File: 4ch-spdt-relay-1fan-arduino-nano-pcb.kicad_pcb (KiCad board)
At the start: 2 copper layers, 143.9 x 97.2 mm, 54 parts, among them J1 Screw_Terminal_01x03, J2 Conn_01x08_Pin, J3 Screw_Terminal_01x03, J4 Screw_Terminal_01x03, J5 Screw_Terminal_01x03, J7 Conn_01x07_Pin, J9 Conn_01x04_Pin, K1 G5LE-1, K2 G5LE-1, K3 G5LE-1, K4 G5LE-1, Q1 2N3904, Q2 2N3904, Q3 2N3904, Q4 2N3904, Q5 BT136, U5 MOC3021M, U6 PC817, U7 TSOP1738, U8 HLK-10M05

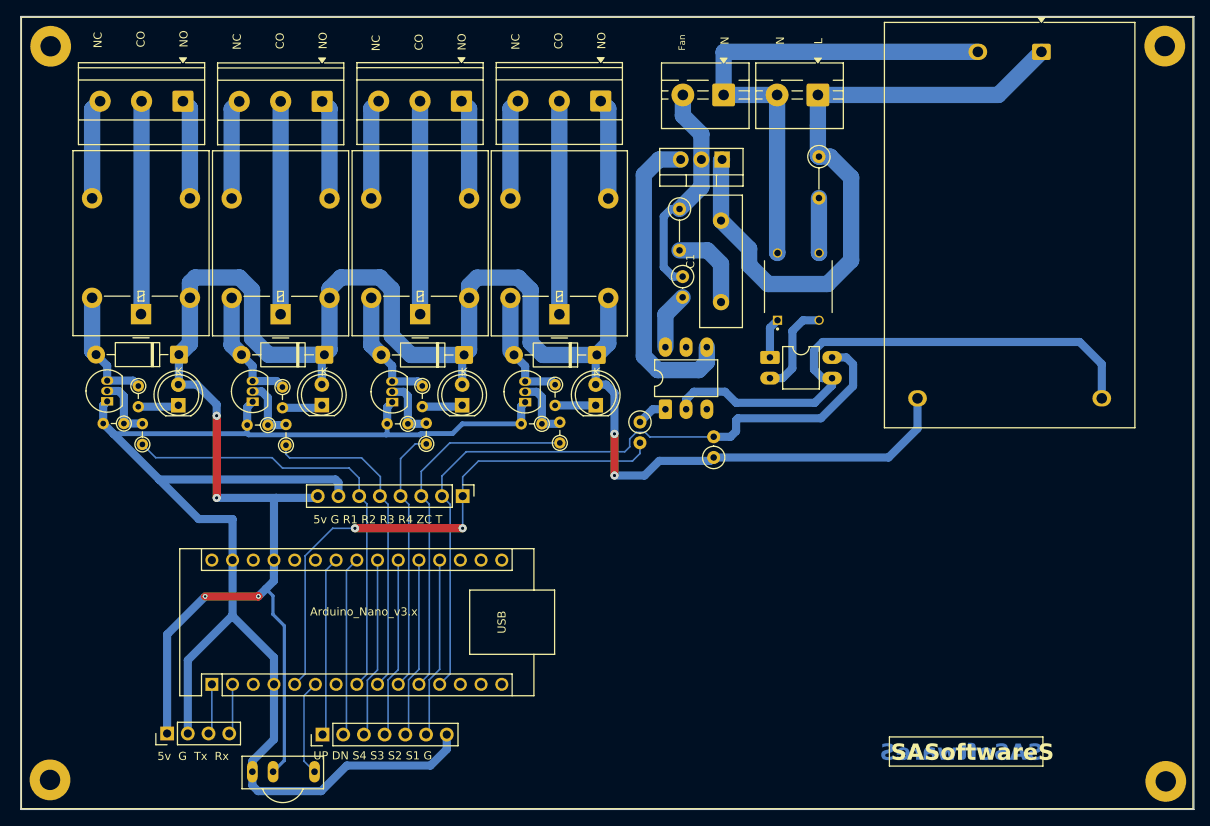
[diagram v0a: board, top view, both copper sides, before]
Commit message: Add files via upload
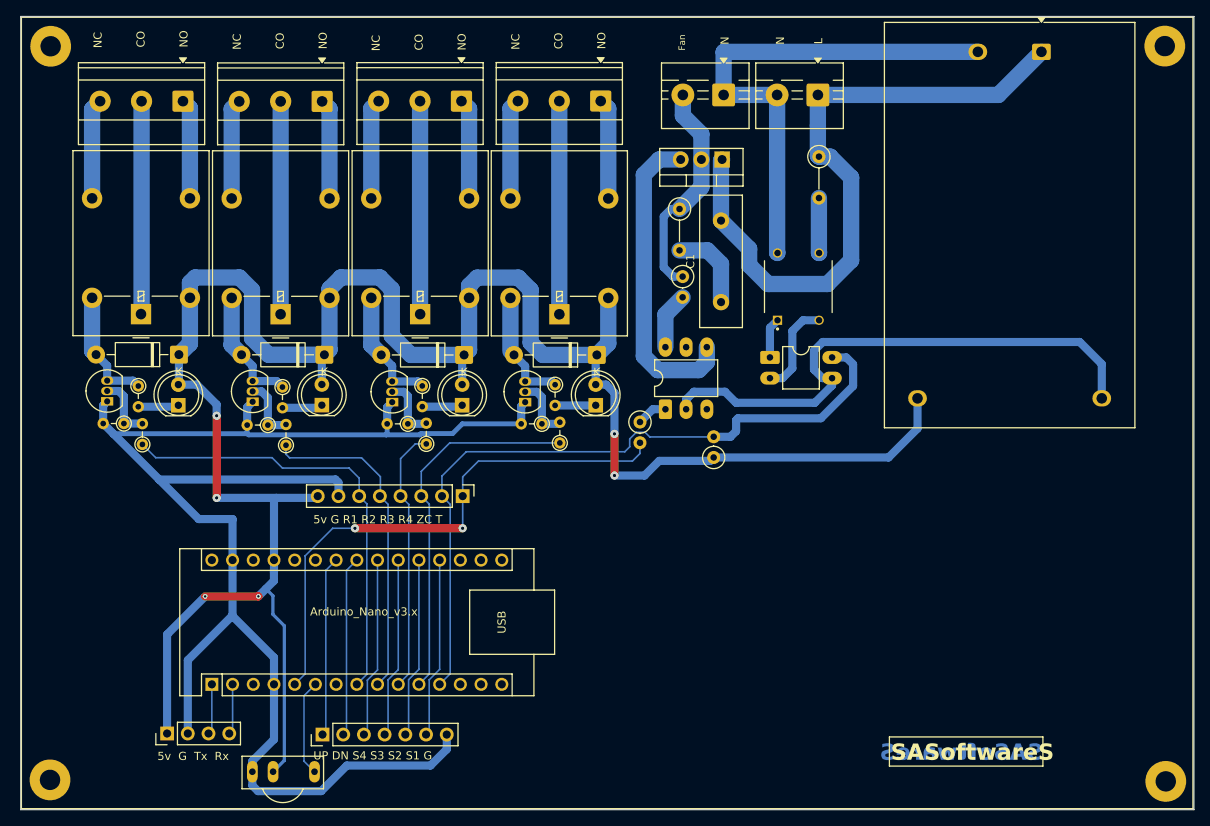
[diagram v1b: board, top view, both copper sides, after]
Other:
- board size 143.9 x 97.2 mm -> 143.9 x 97.3 mm
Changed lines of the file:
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@@
 		(model "${KICAD10_3DMODEL_DIR}/Module.3dshapes/Arduino_Nano.STEP"
 			(offset
-				(xyz 7.5 -17.5 0)
+				(xyz 7.63 -17.8 0)
 			)
 			(scale
@@
 	(gr_rect
 		(start 80.35 54.74)
-		(end 224.24 151.99)
+		(end 224.24 152.02)
 		(stroke
 			(width 0.05)

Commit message: Add files via upload
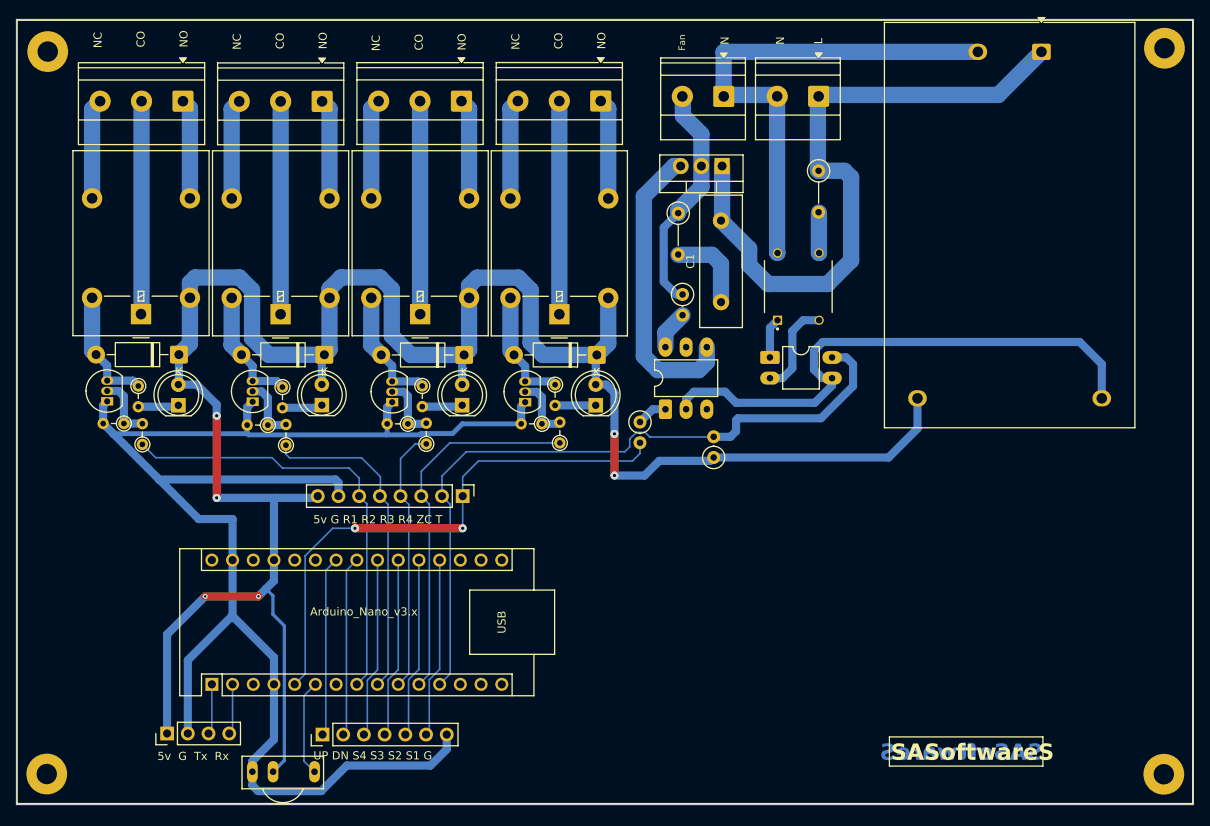
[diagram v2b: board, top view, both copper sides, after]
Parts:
- J6, J8: footprint TerminalBlock:TerminalBlock_MaiXu_MX126-5.0-02P_1x02_P5.00mm -> TerminalBlock_Phoenix:TerminalBlock_Phoenix_MKDS-1,5-2-5.08_1x02_P5.08mm_Horizontal
- moved R19 2.20 mm to (161.5, 88.8)
- moved R18 1.74 mm to (178.2, 73.7)
- moved REF** 0.90 mm to (220.6, 147.7)
- moved REF** 0.82 mm to (83.5, 147.7)
- moved Q5 0.80 mm to (166.4, 73.1)
- moved REF** 0.74 mm to (83.7, 59.0)
- moved R20 0.53 mm to (161.0, 78.9)
- moved REF** 0.26 mm to (220.6, 58.6)
- moved J6 0.19 mm to (178.2, 64.5)
- moved J8 0.18 mm to (166.6, 64.5)
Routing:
- net Net-(R19-Pad2): track 6.98 -> 4.78 mm
- net Net-(Q5-G): track 38.2 -> 36.3 mm
- net Net-(BR1-Pad3): track 6.75 -> 4.97 mm
- net Net-(J8-Pin_2): track 27.4 -> 28.7 mm
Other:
- board size 143.9 x 97.3 mm -> 144.3 x 96.3 mm
